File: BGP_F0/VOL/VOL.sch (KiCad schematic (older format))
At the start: 4 parts, among them J1 Conn_01x03_Female, J2 Conn_01x03_Female, P1 CONN_01X02

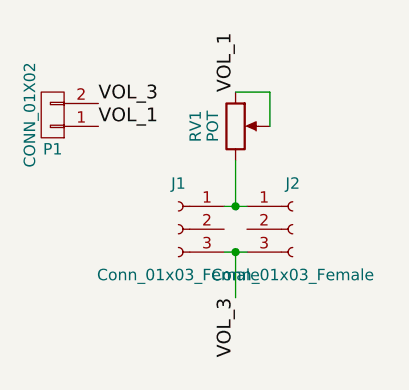
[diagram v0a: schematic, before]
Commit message: Mid Buff
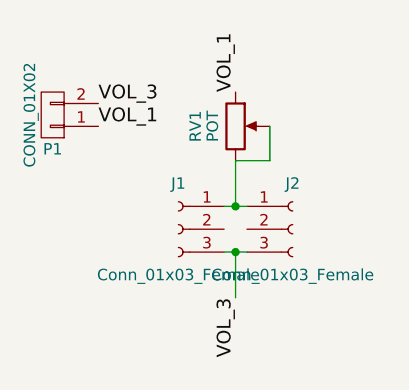
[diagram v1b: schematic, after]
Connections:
- net VOL_1: no longer RV1.2
- net at J1.1 (Pin_1), J2.1 (Pin_1), RV1.3: now also RV1.2
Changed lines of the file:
@@
 Text Label 5800 3050 1    60   ~ 0
 VOL_1
-Wire Wire Line
-	5800 3050 5950 3050
-Wire Wire Line
-	5950 3050 5950 3200
 $Comp
 L CONN_01X02 P1
@@
 	5800 3750 5800 3950
 Connection ~ 5800 3750
+Wire Wire Line
+	5950 3200 5950 3350
+Wire Wire Line
+	5950 3350 5800 3350
 $EndSCHEMATC
